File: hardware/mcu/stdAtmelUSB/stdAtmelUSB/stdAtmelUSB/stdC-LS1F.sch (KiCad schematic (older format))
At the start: 1 part

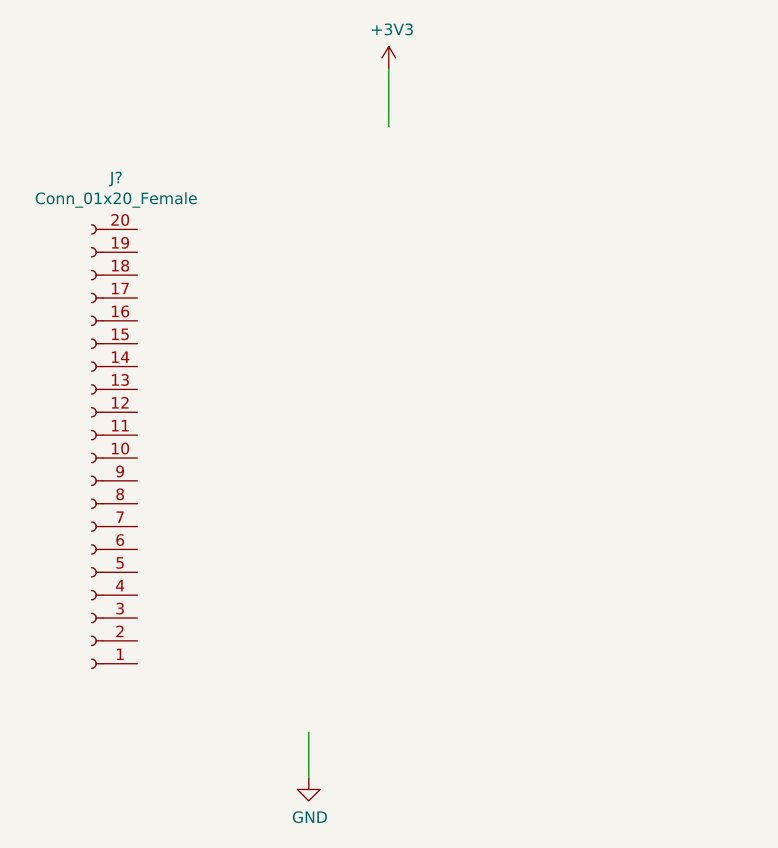
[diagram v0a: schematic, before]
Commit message: std boards skeletons
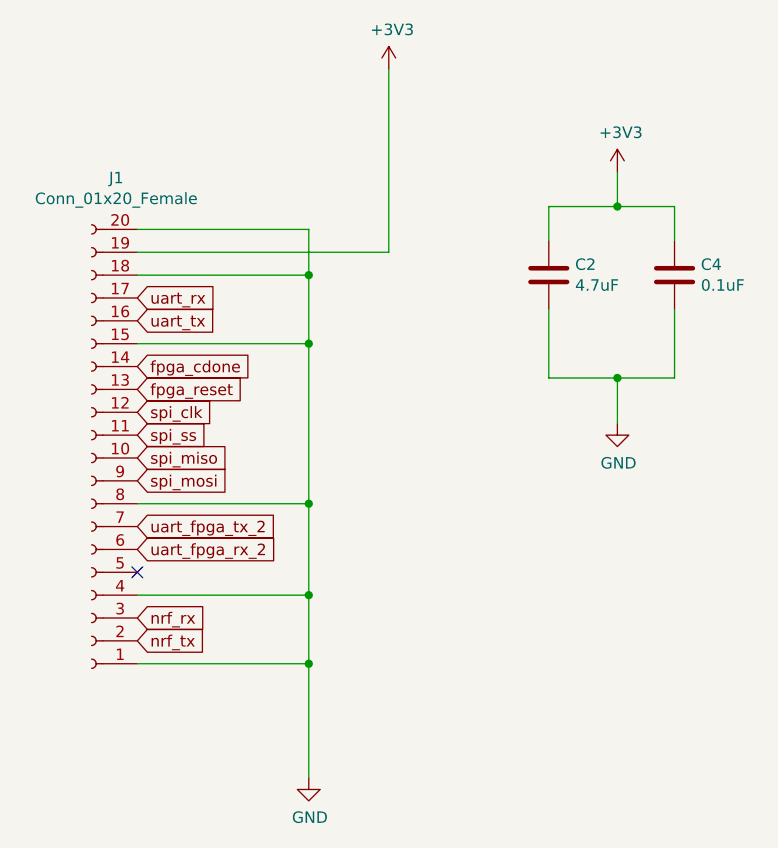
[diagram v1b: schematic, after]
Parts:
- added C2: 4.7uF, Capacitor_SMD:C_0402_1005Metric, symbol Device:C
- added C4: 0.1uF, Capacitor_SMD:C_0402_1005Metric, symbol Device:C
- J1: renamed from J?; footprint (none) -> Connector_PinHeader_2.54mm:PinHeader_1x20_P2.54mm_Horizontal
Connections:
- net labels added: fpga_cdone, fpga_reset, nrf_rx, nrf_tx, spi_clk, spi_miso, spi_mosi, spi_ss, uart_fpga_rx_2, uart_fpga_tx_2, uart_rx, uart_tx
- wire segments 2 -> 24
- no-connect marks 0 -> 1
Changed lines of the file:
@@
 $EndDescr
 $Comp
-L Connector:Conn_01x20_Female J?
+L Connector:Conn_01x20_Female J1
 U 1 1 5E9E9075
 P 2050 3500
-F 0 "J?" H 1942 2275 50  0000 C CNN
+F 0 "J1" H 1942 2275 50  0000 C CNN
 F 1 "Conn_01x20_Female" H 1942 2366 50  0000 C CNN
-F 2 "" H 2050 3500 50  0001 C CNN
+F 2 "Connector_PinHeader_2.54mm:PinHeader_1x20_P2.54mm_Horizontal" H 2050 3500 50  0001 C CNN
 F 3 "~" H 2050 3500 50  0001 C CNN
 	1    2050 3500
@@
 P 3350 1800
 AR Path="/5E9E6BE4/5E9ECCA0" Ref="#PWR?"  Part="1"
-AR Path="/5E9E8D09/5E9ECCA0" Ref="#PWR?"  Part="1"
-F 0 "#PWR?" H 3350 1650 50  0001 C CNN
+AR Path="/5E9E8D09/5E9ECCA0" Ref="#PWR04"  Part="1"
+F 0 "#PWR04" H 3350 1650 50  0001 C CNN
 F 1 "+3V3" H 3365 1973 50  0000 C CNN
 F 2 "" H 3350 1800 50  0001 C CNN
@@
 	1    0    0    -1
 $EndComp
-Wire Wire Line
-	3350 1800 3350 2050
 $Comp
-L power:GND #PWR?
+L power:GND #PWR03
 U 1 1 5E9EE351
 P 3000 4900
-F 0 "#PWR?" H 3000 4650 50  0001 C CNN
+F 0 "#PWR03" H 3000 4650 50  0001 C CNN
 F 1 "GND" H 3005 4727 50  0000 C CNN
 F 2 "" H 3000 4900 50  0001 C CNN
@@
 	1    0    0    -1
 $EndComp
+Text GLabel 2250 2900 2    50   Input ~ 0
+uart_tx
+Text GLabel 2250 2800 2    50   Input ~ 0
+uart_rx
+Text GLabel 2250 3300 2    50   Input ~ 0
+spi_clk
+Text GLabel 2250 3400 2    50   Input ~ 0
+spi_ss
+Text GLabel 2250 3500 2    50   Input ~ 0
+spi_miso
+Text GLabel 2250 3600 2    50   Input ~ 0
+spi_mosi
+Text GLabel 2250 3200 2    50   Input ~ 0
+fpga_reset
+Text GLabel 2250 3100 2    50   Input ~ 0
+fpga_cdone
+Text GLabel 2250 3800 2    50   Input ~ 0
+uart_fpga_tx_2
+Text GLabel 2250 3900 2    50   Input ~ 0
+uart_fpga_rx_2
+Text GLabel 2250 4200 2    50   Input ~ 0
+nrf_rx
+Text GLabel 2250 4300 2    50   Input ~ 0
+nrf_tx
+$Comp
+L Device:C C?
+U 1 1 5E9F19A3
+P 4600 2700
+AR Path="/5E9E6BB8/5E9F19A3" Ref="C?"  Part="1"
+AR Path="/5E9E8D09/5E9F19A3" Ref="C4"  Part="1"
+F 0 "C4" H 4715 2746 50  0000 L CNN
+F 1 "0.1uF" H 4715 2655 50  0000 L CNN
+F 2 "Capacitor_SMD:C_0402_1005Metric" H 4638 2550 50  0001 C CNN
+F 3 "~" H 4600 2700 50  0001 C CNN
+	1    4600 2700
+	1    0    0    -1
+$EndComp
+$Comp
+L Device:C C?
+U 1 1 5E9F19A9
+P 4050 2700
+AR Path="/5E9E6BB8/5E9F19A9" Ref="C?"  Part="1"
+AR Path="/5E9E8D09/5E9F19A9" Ref="C2"  Part="1"
+F 0 "C2" H 4165 2746 50  0000 L CNN
+F 1 "4.7uF" H 4165 2655 50  0000 L CNN
+F 2 "Capacitor_SMD:C_0402_1005Metric" H 4088 2550 50  0001 C CNN
+F 3 "~" H 4050 2700 50  0001 C CNN
+	1    4050 2700
+	1    0    0    -1
+$EndComp
+$Comp
+L power:GND #PWR?
+U 1 1 5E9F19AF
+P 4350 3350
+AR Path="/5E9E6BB8/5E9F19AF" Ref="#PWR?"  Part="1"
+AR Path="/5E9E8D09/5E9F19AF" Ref="#PWR06"  Part="1"
+F 0 "#PWR06" H 4350 3100 50  0001 C CNN
+F 1 "GND" H 4355 3177 50  0000 C CNN
+F 2 "" H 4350 3350 50  0001 C CNN
+F 3 "" H 4350 3350 50  0001 C CNN
+	1    4350 3350
+	1    0    0    -1
+$EndComp
+$Comp
+L power:+3V3 #PWR?
+U 1 1 5E9F19B5
+P 4350 2250
+AR Path="/5E9E6BB8/5E9F19B5" Ref="#PWR?"  Part="1"
+AR Path="/5E9E8D09/5E9F19B5" Ref="#PWR05"  Part="1"
+F 0 "#PWR05" H 4350 2100 50  0001 C CNN
+F 1 "+3V3" H 4365 2423 50  0000 C CNN
+F 2 "" H 4350 2250 50  0001 C CNN
+F 3 "" H 4350 2250 50  0001 C CNN
+	1    4350 2250
+	1    0    0    -1
+$EndComp
 Wire Wire Line
-	3000 4900 3000 4700
+	4050 2850 4050 3150
+Wire Wire Line
+	4050 3150 4350 3150
+Wire Wire Line
+	4600 3150 4600 2850
+Wire Wire Line
+	4050 2550 4050 2400
+Wire Wire Line
+	4050 2400 4350 2400
+Wire Wire Line
+	4600 2400 4600 2550
+Wire Wire Line
+	4350 2250 4350 2400
+Connection ~ 4350 2400
+Wire Wire Line
+	4350 2400 4600 2400
+Wire Wire Line
+	4350 3350 4350 3150
+Connection ~ 4350 3150
+Wire Wire Line
+	4350 3150 4600 3150
+Wire Wire Line
+	2250 2500 3000 2500
+Wire Wire Line
+	3000 2500 3000 2700
+Wire Wire Line
+	2250 2600 3350 2600
+Wire Wire Line
+	3350 1800 3350 2600
+Connection ~ 3000 2700
+Wire Wire Line
+	3000 2700 3000 3000
+Wire Wire Line
+	2250 2700 3000 2700
+Wire Wire Line
+	2250 4400 3000 4400
+Connection ~ 3000 4400
+Wire Wire Line
+	3000 4400 3000 4900
+Wire Wire Line
+	2250 4100 3000 4100
+Connection ~ 3000 4100
+Wire Wire Line
+	3000 4100 3000 4400
+Wire Wire Line
+	2250 3700 3000 3700
+Connection ~ 3000 3700
+Wire Wire Line
+	3000 3700 3000 4100
+NoConn ~ 2250 4000
+Wire Wire Line
+	2250 3000 3000 3000
+Connection ~ 3000 3000
+Wire Wire Line
+	3000 3000 3000 3700
 $EndSCHEMATC
